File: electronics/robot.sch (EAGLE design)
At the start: 57 parts, among them J1 USB-B, J2 DC21MMX, J3 B6B-ZR, J4 B6B-ZR, J5 B6B-ZR, J6 KICKER, Q1 IRLMS2002TRPBF, Q2 IRLMS2002TRPBF, Q3 NPN_BC817,215, Q4 SUD50N04-8M8P-4GE3, U1 FT232L, U2 ESP32-WROOM-32E_(16MB), U3 S8252, U4 L9110, U5 L9110, U6 L9110, U7 MT3608

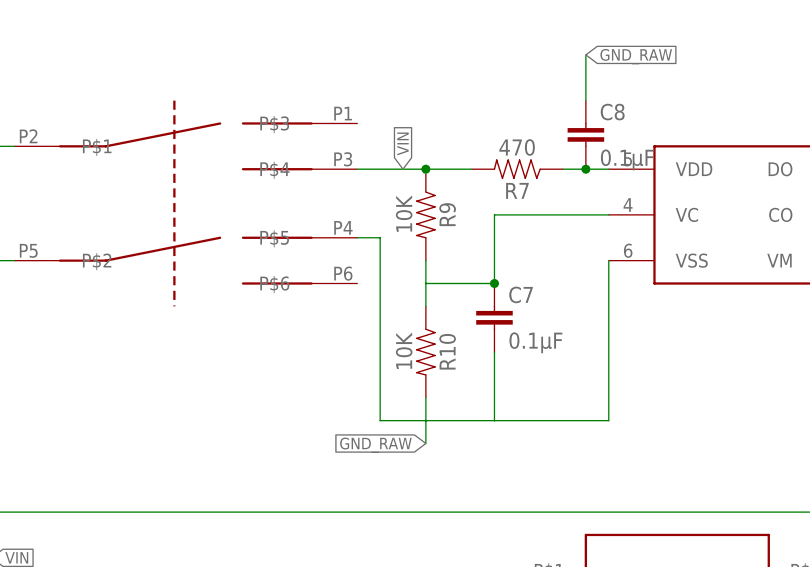
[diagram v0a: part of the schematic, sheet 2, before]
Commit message: BMS resistors
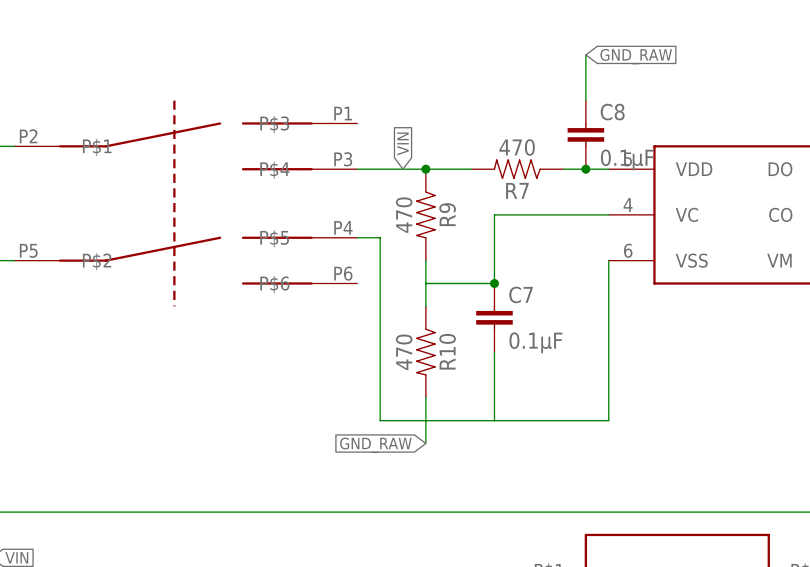
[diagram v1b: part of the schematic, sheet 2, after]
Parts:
- R10, R9: value 10K -> 470
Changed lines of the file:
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@@
 <attribute name="FARNELL" value="2447662"/>
 </part>
-<part name="R9" library="SparkFun-Resistors" deviceset="0.3OHM" device="-0805-1/8W-1%" value="10K">
+<part name="R9" library="SparkFun-Resistors" deviceset="0.3OHM" device="-0805-1/8W-1%" value="470">
 <attribute name="FARNELL" value="2074334RL"/>
 </part>
-<part name="R10" library="SparkFun-Resistors" deviceset="0.3OHM" device="-0805-1/8W-1%" value="10K">
+<part name="R10" library="SparkFun-Resistors" deviceset="0.3OHM" device="-0805-1/8W-1%" value="470">
 <attribute name="FARNELL" value="2074334RL"/>
 </part>
